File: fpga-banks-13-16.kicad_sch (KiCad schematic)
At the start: 40 parts, among them U14 XC7A100T-FGG484, U15 Oscillator_100MHz_AMJMEFB

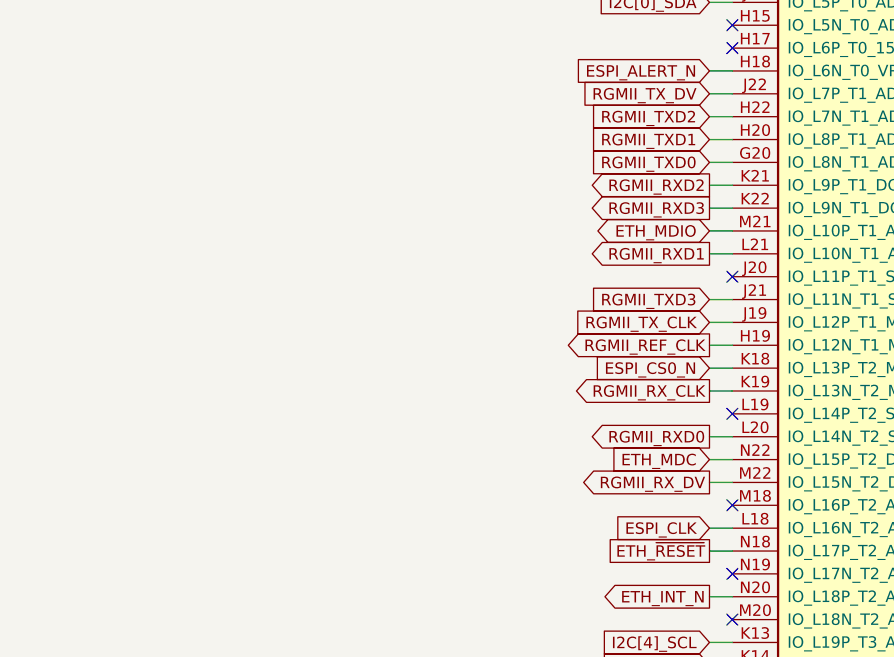
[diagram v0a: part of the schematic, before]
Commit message: pcb layout progress
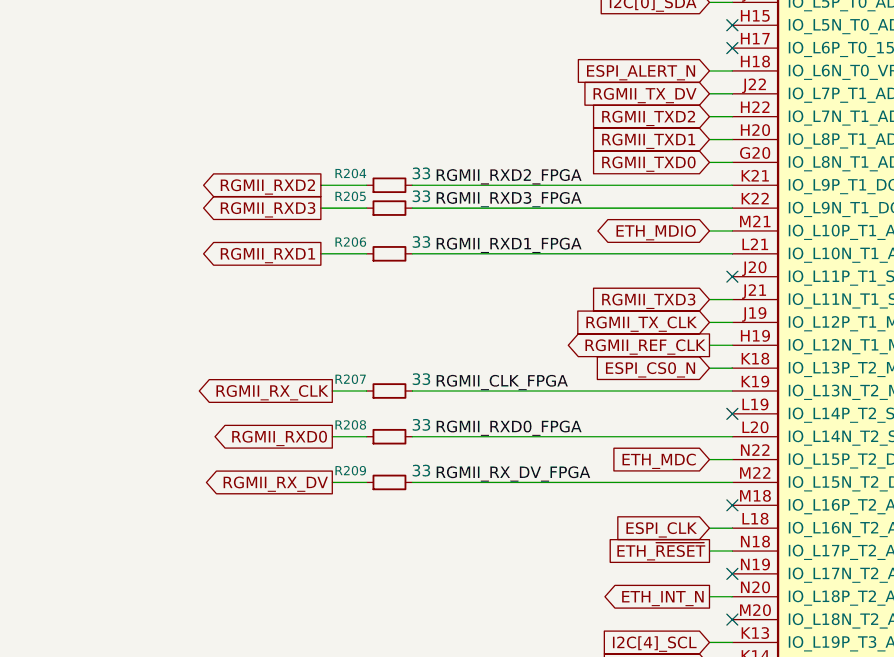
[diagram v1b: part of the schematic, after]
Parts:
- added R204, R205, R206, R207, R208, R209: 33, Resistor_SMD:R_0402_1005Metric, symbol Device:R_Small
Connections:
- net RGMII_RXD0: now also R208.1; no longer U14.L20 (IO_L14N_T2_SRCC_15)
- net RGMII_RXD1: now also R206.1; no longer U14.L21 (IO_L10N_T1_AD11N_15)
- net RGMII_RXD2: now also R204.1; no longer U14.K21 (IO_L9P_T1_DQS_AD3P_15)
- net RGMII_RXD3: now also R205.1; no longer U14.K22 (IO_L9N_T1_DQS_AD3N_15)
- net RGMII_RX_CLK: now also R207.1; no longer U14.K19 (IO_L13N_T2_MRCC_15)
- net RGMII_RX_DV: now also R209.1; no longer U14.M22 (IO_L15N_T2_DQS_ADV_B_15)
- new net RGMII_CLK_FPGA: R207.2, U14.K19 (IO_L13N_T2_MRCC_15)
- new net RGMII_RXD0_FPGA: R208.2, U14.L20 (IO_L14N_T2_SRCC_15)
- new net RGMII_RXD1_FPGA: R206.2, U14.L21 (IO_L10N_T1_AD11N_15)
- new net RGMII_RXD2_FPGA: R204.2, U14.K21 (IO_L9P_T1_DQS_AD3P_15)
- new net RGMII_RXD3_FPGA: R205.2, U14.K22 (IO_L9N_T1_DQS_AD3N_15)
- new net RGMII_RX_DV_FPGA: R209.2, U14.M22 (IO_L15N_T2_DQS_ADV_B_15)
